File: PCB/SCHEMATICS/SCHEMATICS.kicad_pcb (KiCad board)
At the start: 2 copper layers, 100 x 100 mm, 100 parts, among them IC1 CP2102-GMR, J1 Conn_01x24_Pin, J2 Conn_01x24_Pin, Q1 PMOS, U1 C7433, U3 LTR-303ALS-01, U5 LTR-303ALS-01, U6 C6482, U7 C6482

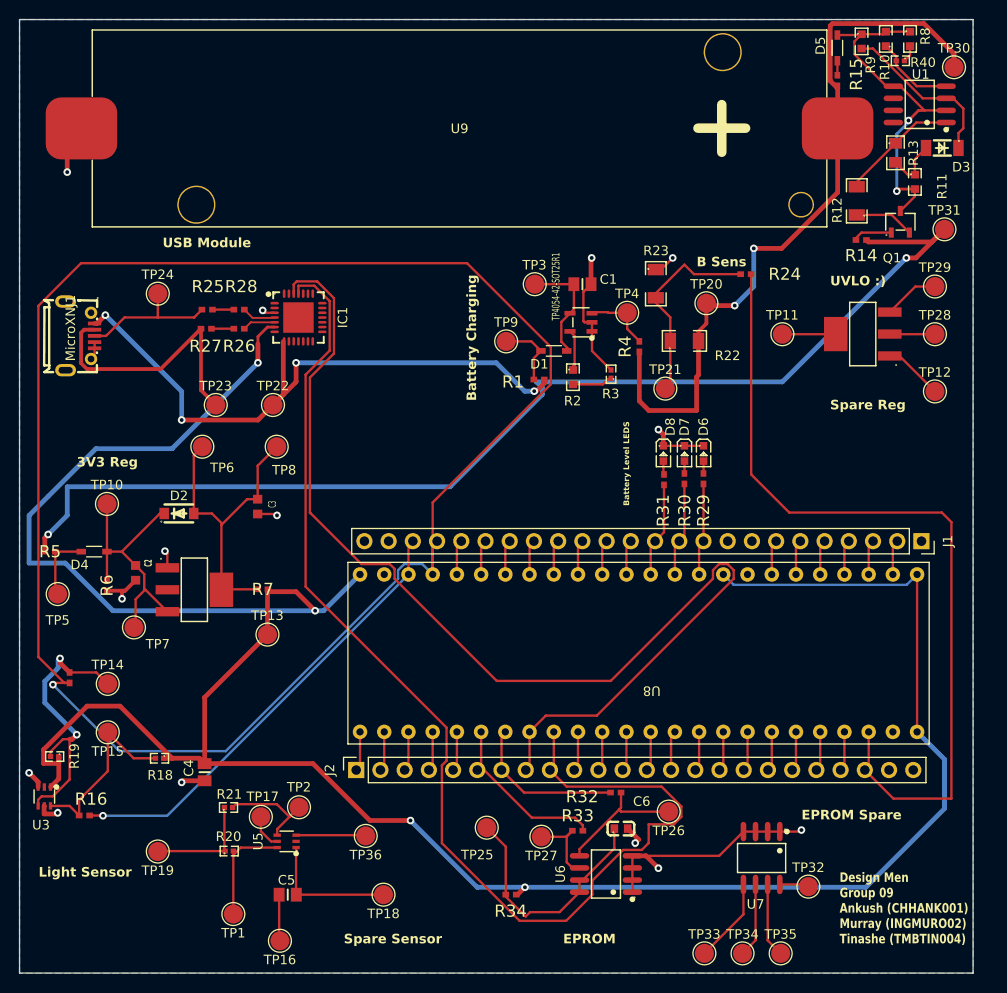
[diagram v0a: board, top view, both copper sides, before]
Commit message: Updating PCB
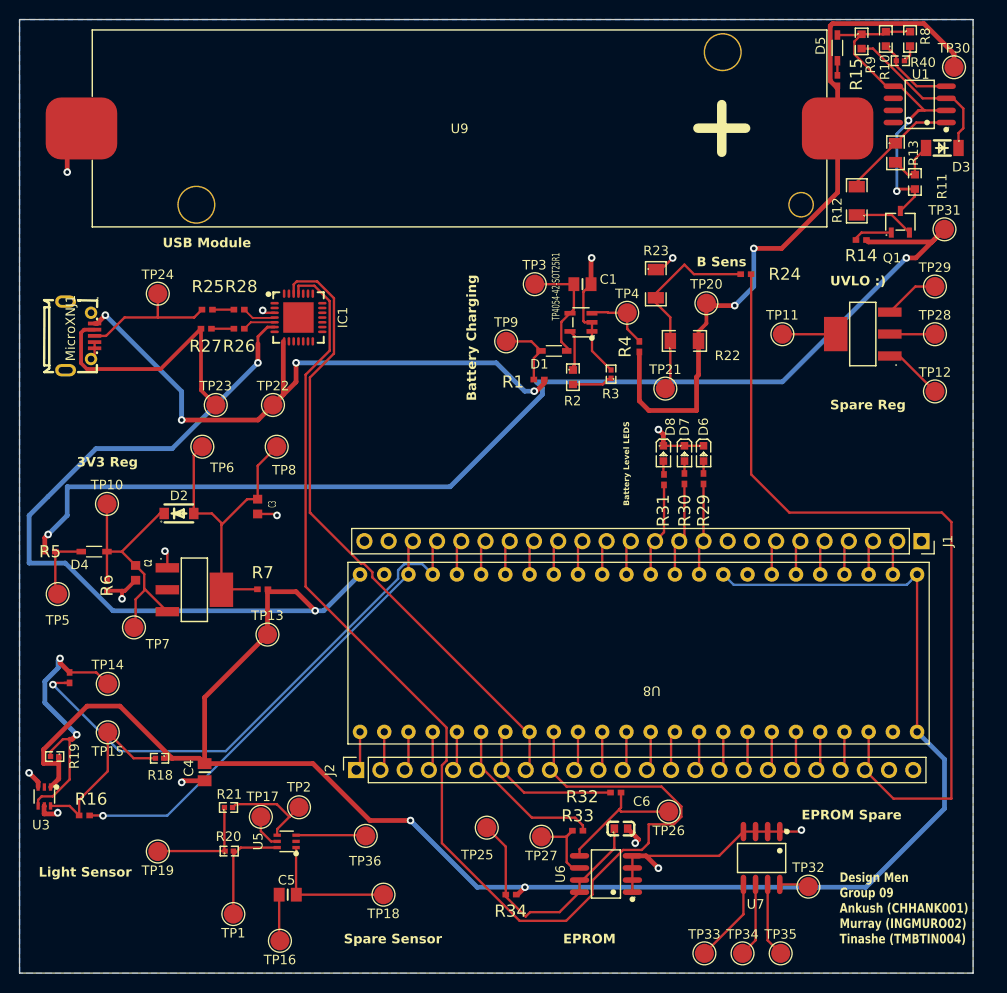
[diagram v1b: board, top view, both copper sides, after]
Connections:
- TP25 pad : (no net) -> Net-(U6-VCC)
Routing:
- net /MICROCONTROLLER/PB10: track 187.0 -> 58.1 mm
- net /MICROCONTROLLER/PA11: track 121.0 -> 66.8 mm
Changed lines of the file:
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@@
     (property "ki_keywords" "test point tp")
     (attr exclude_from_pos_files)
-    (fp_text reference "TP36" (at 0 -1.998) (layer "F.SilkS")
+    (fp_text reference "TP36" (at 0.056274 -2.637967) (layer "F.SilkS")
         (effects (font (size 1 1) (thickness 0.15)))
     )
@@
         (effects (font (size 1 1) (thickness 0.15)))
     )
-    (fp_text user "${REFERENCE}" (at 0 -2) (layer "F.Fab")
+    (fp_text user "${REFERENCE}" (at 0.056274 -2.637967) (layer "F.Fab")
         (effects (font (size 1 1) (thickness 0.15)))
     )
@@
     (property "ki_keywords" "r resistor")
     (attr smd)
-    (fp_text reference "R7" (at 0 0) (layer "F.SilkS")
+    (fp_text reference "R7" (at 0 -1.75) (layer "F.SilkS")
         (effects (font (size 1.27 1.27) (thickness 0.254)))
     )
@@
         (effects (font (size 1.27 1.27) (thickness 0.254)))
     )
-    (fp_text user "${REFERENCE}" (at 0 0) (layer "F.Fab")
+    (fp_text user "${REFERENCE}" (at 0 -1.75) (layer "F.Fab")
         (effects (font (size 1.27 1.27) (thickness 0.254)))
     )
@@
     (fp_circle (center 0 0) (end 1.5 0)
       (stroke (width 0.05) (type solid)) (fill none) (layer "F.CrtYd"))
-    (pad "" smd circle (at 0 0 180) (size 2 2) (layers "F.Cu"))
+    (pad "" smd circle (at 0 0 180) (size 2 2) (layers "F.Cu")
+      (net 16 "Net-(U6-VCC)"))
   )
   (footprint "footprint:RESC1005X40N" (layer "F.Cu")
@@
     (fp_arc (start 1.080188 -0.709627) (mid 1.299286 -0.618875) (end 1.390018 -0.399772)
       (stroke (width 0.254) (type solid)) (layer "F.SilkS"))
-    (fp_arc (start 1.390018 0.400203) (mid 1.299267 0.61928) (end 1.080188 0.710033)
+    (fp_arc (start 1.390018 0.400203) (mid 1.299267 0.619284) (end 1.080188 0.710033)
       (stroke (width 0.254) (type solid)) (layer "F.SilkS"))
     (fp_circle (center -0.800102 0.400051) (end -0.77013 0.400051)
@@
         (effects (font (size 1 1) (thickness 0.15)))
     )
-    (fp_text value "3M" (at 0 1.786634 90) (layer "F.Fab")
+    (fp_text value "3M" (at -1.029366 -2.862 90) (layer "F.Fab")
         (effects (font (size 1 1) (thickness 0.15)))
     )
@@
         (effects (font (size 1 1) (thickness 0.15)))
     )
-    (fp_text user "${REFERENCE}" (at 0 -2) (layer "F.Fab")
+    (fp_text user "${REFERENCE}" (at 0 2.112033) (layer "F.Fab")
         (effects (font (size 1 1) (thickness 0.15)))
     )
@@
   (segment (start 133.3265 103.3235) (end 133.3265 106.1935) (width 0.25) (layer "F.Cu") (net 28))
   (segment (start 93.68 117.57) (end 93.5 117.75) (width 0.25) (layer "F.Cu") (net 28))
-  (segment (start 136.930302 73.55) (end 145.70884 82.328538) (width 0.25) (layer "F.Cu") (net 28))
-  (segment (start 145.70884 82.328538) (end 145.70884 86.264934) (width 0.25) (layer "F.Cu") (net 28))
-  (segment (start 145.70884 86.264934) (end 133.3265 98.647274) (width 0.25) (layer "F.Cu") (net 28))
   (segment (start 133.7865 102.7035) (end 133.9465 102.7035) (width 0.25) (layer "F.Cu") (net 28))
-  (segment (start 96.45 73.55) (end 136.930302 73.55) (width 0.25) (layer "F.Cu") (net 28))
   (segment (start 95.25 117.57) (end 93.68 117.57) (width 0.25) (layer "F.Cu") (net 28))
-  (segment (start 91.975 78.025) (end 96.45 73.55) (width 0.25) (layer "F.Cu") (net 28))
-  (segment (start 133.3265 98.647274) (end 133.3265 106.1935) (width 0.25) (layer "F.Cu") (net 28))
   (segment (start 95.25 117.57) (end 94.7 117.57) (width 0.25) (layer "F.Cu") (net 28))
-  (segment (start 91.975 114.845) (end 91.975 78.025) (width 0.25) (layer "F.Cu") (net 28))
   (segment (start 133.9465 102.7035) (end 133.3265 103.3235) (width 0.25) (layer "F.Cu") (net 28))
-  (segment (start 94.7 117.57) (end 91.975 114.845) (width 0.25) (layer "F.Cu") (net 28))
   (via (at 93.5 117.75) (size 0.8) (drill 0.4) (layers "F.Cu" "B.Cu") (free) (net 28))
   (segment (start 130.336249 105.1065) (end 132.2395 105.1065) (width 0.25) (layer "B.Cu") (net 28))
@@
   (segment (start 140.5465 123.1035) (end 140.9465 122.7035) (width 0.25) (layer "F.Cu") (net 31))
   (segment (start 142.911504 129.068504) (end 151.978916 129.068504) (width 0.25) (layer "F.Cu") (net 31))
+  (segment (start 120.5 99.75) (end 125.75 105) (width 0.25) (layer "F.Cu") (net 32))
   (segment (start 122.975 83.025) (end 120.45 85.55) (width 0.25) (layer "F.Cu") (net 32))
-  (segment (start 164.256751 105.1065) (end 164.8935 105.743249) (width 0.25) (layer "F.Cu") (net 32))
+  (segment (start 143.2035 122.7035) (end 143.4865 122.7035) (width 0.25) (layer "F.Cu") (net 32))
   (segment (start 118.749492 76.75) (end 118.749492 75.77797) (width 0.25) (layer "F.Cu") (net 32))
-  (segment (start 129.3335 105.618038) (end 129.3335 106.643751) (width 0.25) (layer "F.Cu") (net 32))
-  (segment (start 162.7195 105.743249) (end 163.356249 105.1065) (width 0.25) (layer "F.Cu") (net 32))
-  (segment (start 125.8565 105.1065) (end 128.821962 105.1065) (width 0.25) (layer "F.Cu") (net 32))
-  (segment (start 164.8935 106.643751) (end 150.537251 121) (width 0.25) (layer "F.Cu") (net 32))
-  (segment (start 152.007104 117.3565) (end 162.7195 106.644104) (width 0.25) (layer "F.Cu") (net 32))
+  (segment (start 127 105.949749) (end 127 106.5) (width 0.25) (layer "F.Cu") (net 32))
   (segment (start 120.45 85.55) (end 120.45 99.75) (width 0.25) (layer "F.Cu") (net 32))
-  (segment (start 140.046249 117.3565) (end 152.007104 117.3565) (width 0.25) (layer "F.Cu") (net 32))
-  (segment (start 162.7195 106.644104) (end 162.7195 105.743249) (width 0.25) (layer "F.Cu") (net 32))
   (segment (start 119.063477 75.463985) (end 121.213985 75.463985) (width 0.25) (layer "F.Cu") (net 32))
   (segment (start 121.213985 75.463985) (end 122.975 77.225) (width 0.25) (layer "F.Cu") (net 32))
   (segment (start 143.4865 122.7035) (end 143.4865 126.3035) (width 0.25) (layer "F.Cu") (net 32))
-  (segment (start 129.3335 106.643751) (end 140.046249 117.3565) (width 0.25) (layer "F.Cu") (net 32))
-  (segment (start 163.356249 105.1065) (end 164.256751 105.1065) (width 0.25) (layer "F.Cu") (net 32))
+  (segment (start 125.75 105) (end 126.050251 105) (width 0.25) (layer "F.Cu") (net 32))
   (segment (start 120.45 99.75) (end 120.5 99.75) (width 0.25) (layer "F.Cu") (net 32))
-  (segment (start 150.537251 121) (end 145.19 121) (width 0.25) (layer "F.Cu") (net 32))
-  (segment (start 164.8935 105.743249) (end 164.8935 106.643751) (width 0.25) (layer "F.Cu") (net 32))
+  (segment (start 127 106.5) (end 143.2035 122.7035) (width 0.25) (layer "F.Cu") (net 32))
   (segment (start 118.749492 75.77797) (end 119.063477 75.463985) (width 0.25) (layer "F.Cu") (net 32))
-  (segment (start 145.19 121) (end 143.4865 122.7035) (width 0.25) (layer "F.Cu") (net 32))
-  (segment (start 120.5 99.75) (end 125.8565 105.1065) (width 0.25) (layer "F.Cu") (net 32))
   (segment (start 122.975 77.225) (end 122.975 83.025) (width 0.25) (layer "F.Cu") (net 32))
-  (segment (start 128.821962 105.1065) (end 129.3335 105.618038) (width 0.25) (layer "F.Cu") (net 32))
+  (segment (start 125.75 105) (end 125.8565 105.1065) (width 0.25) (layer "F.Cu") (net 32))
+  (segment (start 126.050251 105) (end 127 105.949749) (width 0.25) (layer "F.Cu") (net 32))
   (segment (start 143.4865 126.3035) (end 143.0865 126.7035) (width 0.25) (layer "F.Cu") (net 32))
   (segment (start 146.0265 122.7035) (end 146.0265 126.3035) (width 0.25) (layer "F.Cu") (net 33))
